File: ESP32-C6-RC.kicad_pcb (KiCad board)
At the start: 2 copper layers, 23 x 32.5 mm, 22 parts, among them J3 Conn_01x03, SW1 SW_Push, U1 ESP32-C6 zero, U2 RZ7899, U3 AMS1117-5.0

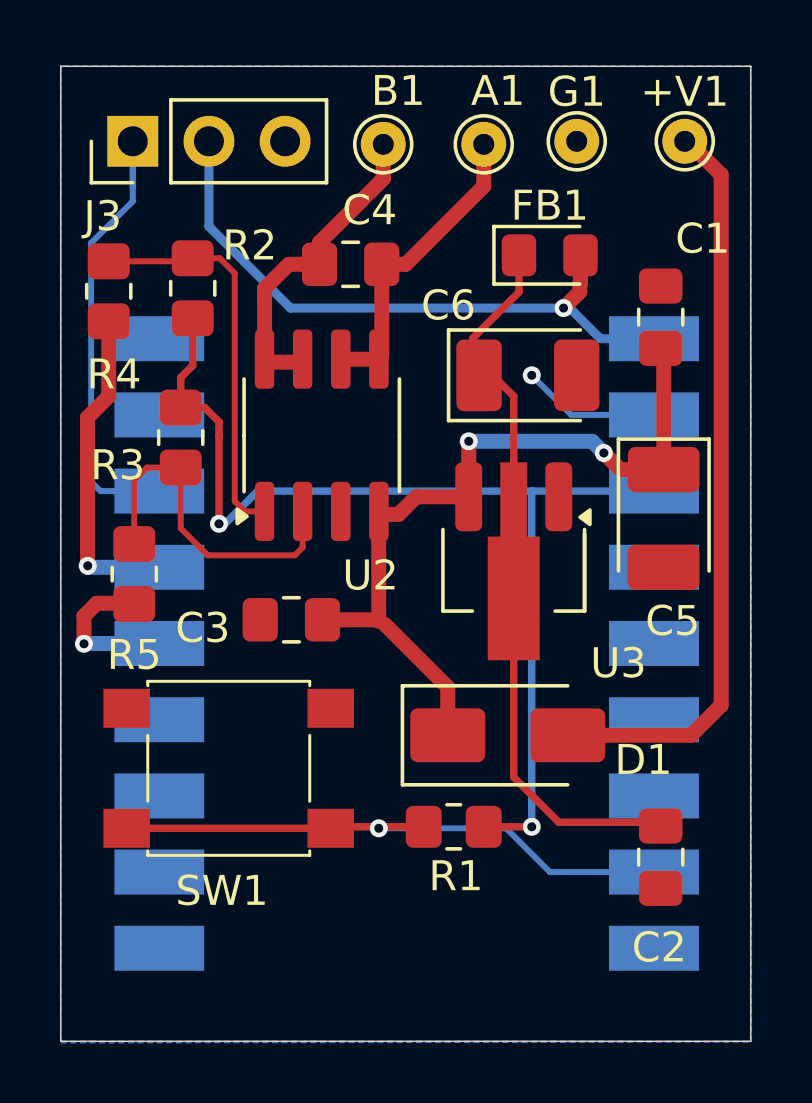
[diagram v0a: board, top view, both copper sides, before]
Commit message: fix pcb
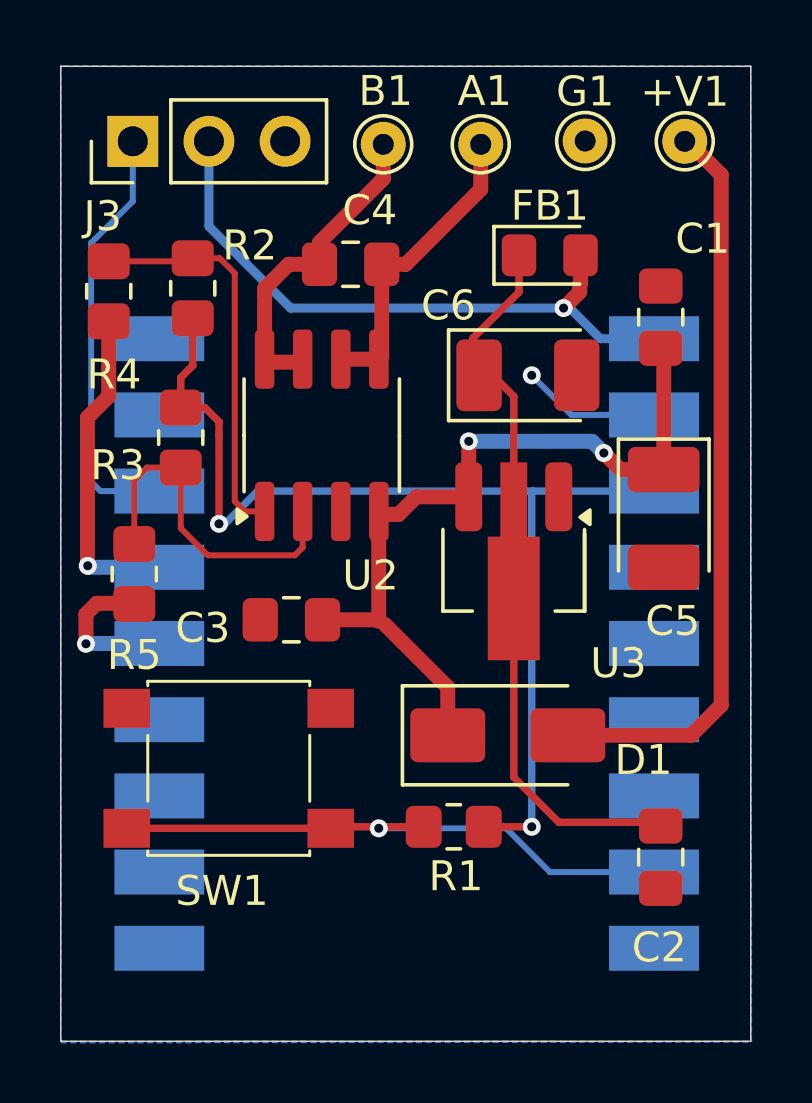
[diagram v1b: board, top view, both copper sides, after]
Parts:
- moved G1 0.28 mm to (90.5, 42.5)
- moved A1 0.10 mm to (87.0, 42.6)
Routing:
- net SERVO_X: track 16.7 -> 15.2 mm
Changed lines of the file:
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@@
 		(tags "test point THT pad")
 		(property "Reference" "B1"
-			(at -0.5 1.775 0)
+			(at -0.08 1.775 0)
 			(layer "F.SilkS")
 			(effects
@@
 	(footprint "TestPoint:TestPoint_THTPad_D1.5mm_Drill0.7mm"
 		(layer "F.Cu")
-		(at 87.1 42.6 180)
+		(at 87 42.6 180)
 		(descr "THT pad as test Point, diameter 1.5mm, hole diameter 0.7mm")
 		(tags "test point THT pad")
 		(property "Reference" "A1"
-			(at -0.475 1.775 0)
+			(at -0.13 1.775 0)
 			(layer "F.SilkS")
 			(effects
@@
 	(footprint "TestPoint:TestPoint_THTPad_D1.5mm_Drill0.7mm"
 		(layer "F.Cu")
-		(at 90.2 42.5)
+		(at 90.48 42.49)
 		(descr "THT pad as test Point, diameter 1.5mm, hole diameter 0.7mm")
 		(tags "test point THT pad")
@@
 	)
 	(segment
-		(start 79.795 47.6)
-		(end 79.795 47.405)
+		(start 83.75 42.6)
+		(end 83.75 43.75)
 		(width 0.5)
 		(layer "F.Cu")
@@
 	)
 	(segment
-		(start 83.75 43.75)
-		(end 83.75 42.6)
+		(start 79.795 47.6)
+		(end 79.795 47.405)
 		(width 0.5)
 		(layer "F.Cu")
@@
 	)
 	(segment
-		(start 87.1 44)
-		(end 87.1 42.6)
+		(start 87 44.1)
+		(end 86.865 44.235)
+		(width 0.5)
+		(layer "F.Cu")
+		(net 5)
+	)
+	(segment
+		(start 87 42.6)
+		(end 87 44.1)
 		(width 0.5)
 		(layer "F.Cu")
@@
 	(segment
 		(start 84.5 46.6)
-		(end 87.1 44)
+		(end 86.865 44.235)
 		(width 0.5)
 		(layer "F.Cu")
@@
 	)
 	(segment
-		(start 75.4 44.075)
-		(end 75.4 42.5)
-		(width 0.2)
-		(layer "B.Cu")
-		(net 8)
-	)
-	(segment
 		(start 74.013 53.848)
 		(end 74.325 54.16)
@@
 	)
 	(segment
-		(start 79.565 54.16)
-		(end 79.6 54.16)
-		(width 0.2)
-		(layer "B.Cu")
-		(net 9)
-	)
-	(segment
 		(start 88.7 54.185)
 		(end 88.725 54.16)
@@
 	)
 	(segment
-		(start 73.775 58.325)
-		(end 74.2 57.9)
+		(start 73.84 59.25)
+		(end 73.84 58.26)
 		(width 0.5)
 		(layer "F.Cu")
@@
 	)
 	(segment
-		(start 73.775 59.25)
-		(end 73.775 58.325)
+		(start 75.1 57.9)
+		(end 75.2 57.8)
 		(width 0.5)
 		(layer "F.Cu")
@@
 	)
 	(segment
-		(start 75.1 57.9)
-		(end 75.2 57.8)
+		(start 74.2 57.9)
+		(end 75.1 57.9)
 		(width 0.5)
 		(layer "F.Cu")
@@
 	)
 	(segment
-		(start 74.2 57.9)
-		(end 75.1 57.9)
+		(start 73.84 58.26)
+		(end 74.2 57.9)
 		(width 0.5)
 		(layer "F.Cu")
@@
 	)
 	(via
-		(at 73.775 59.25)
+		(at 73.84 59.25)
 		(size 0.6)
 		(drill 0.3)
